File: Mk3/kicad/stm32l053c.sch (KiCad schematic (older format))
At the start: 24 parts, among them J1 CONN_01X02, P1 SWD, U1 AP2112, U2 STM32L053C8_LQFP48, U3 ADS1015, U4 EDGE_SMA, U5 RFM92/95

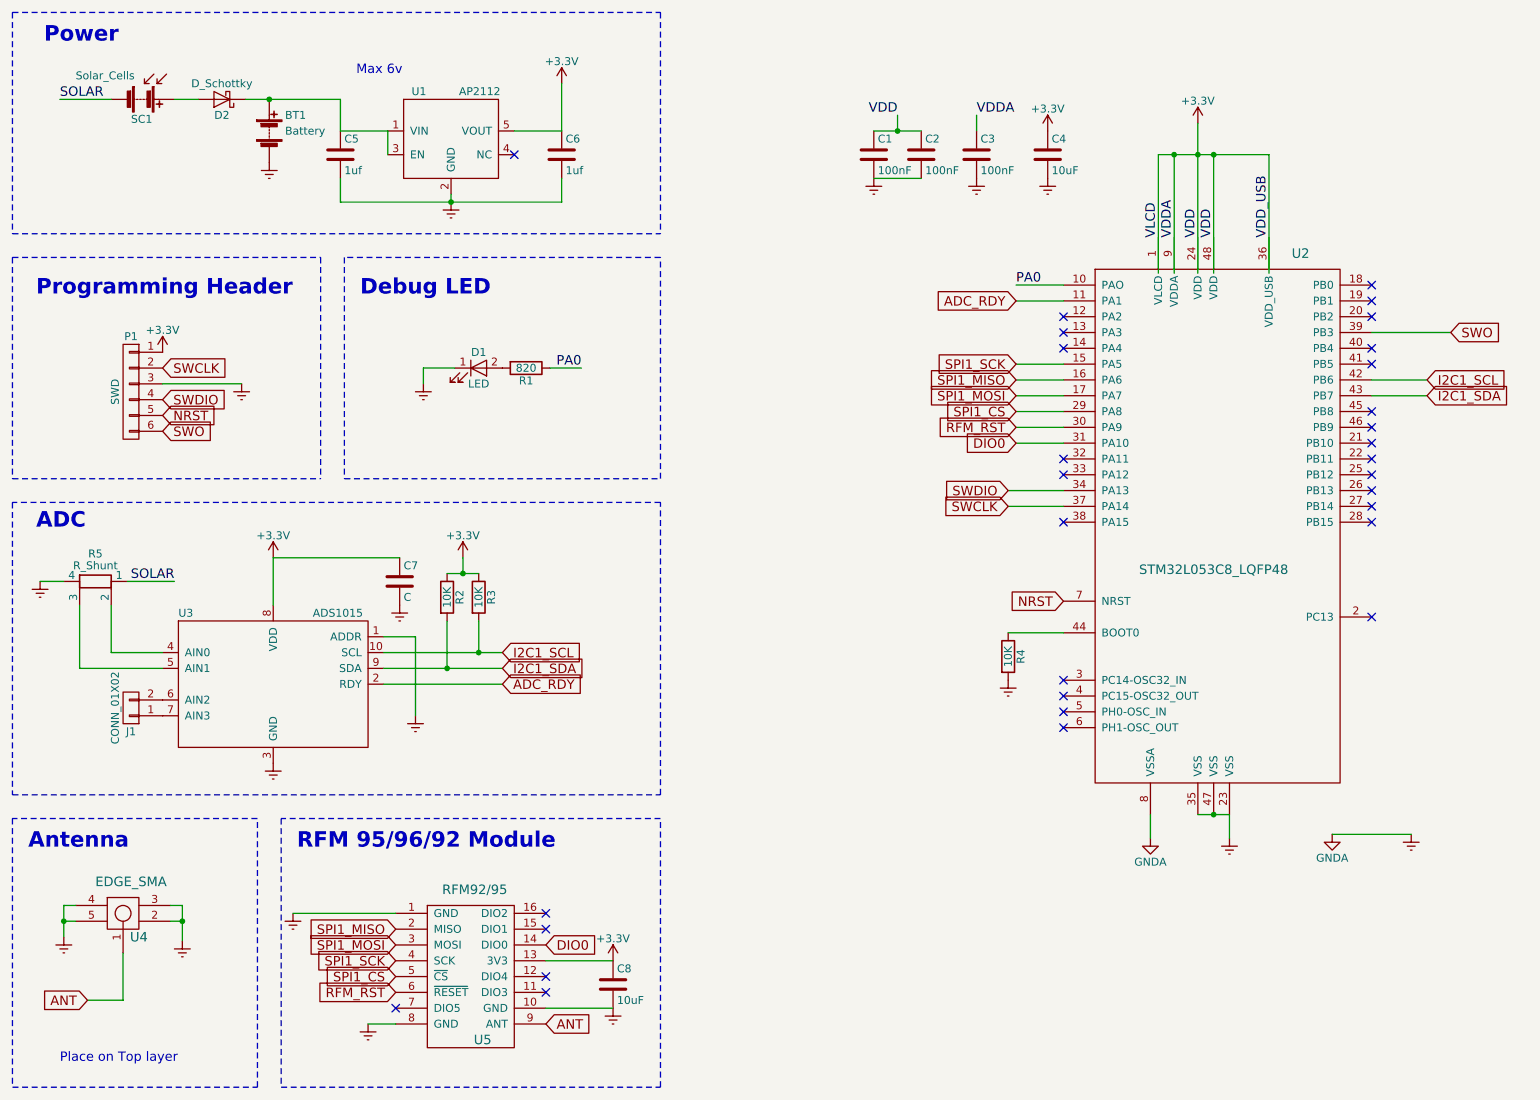
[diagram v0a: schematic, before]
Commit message: Solar power
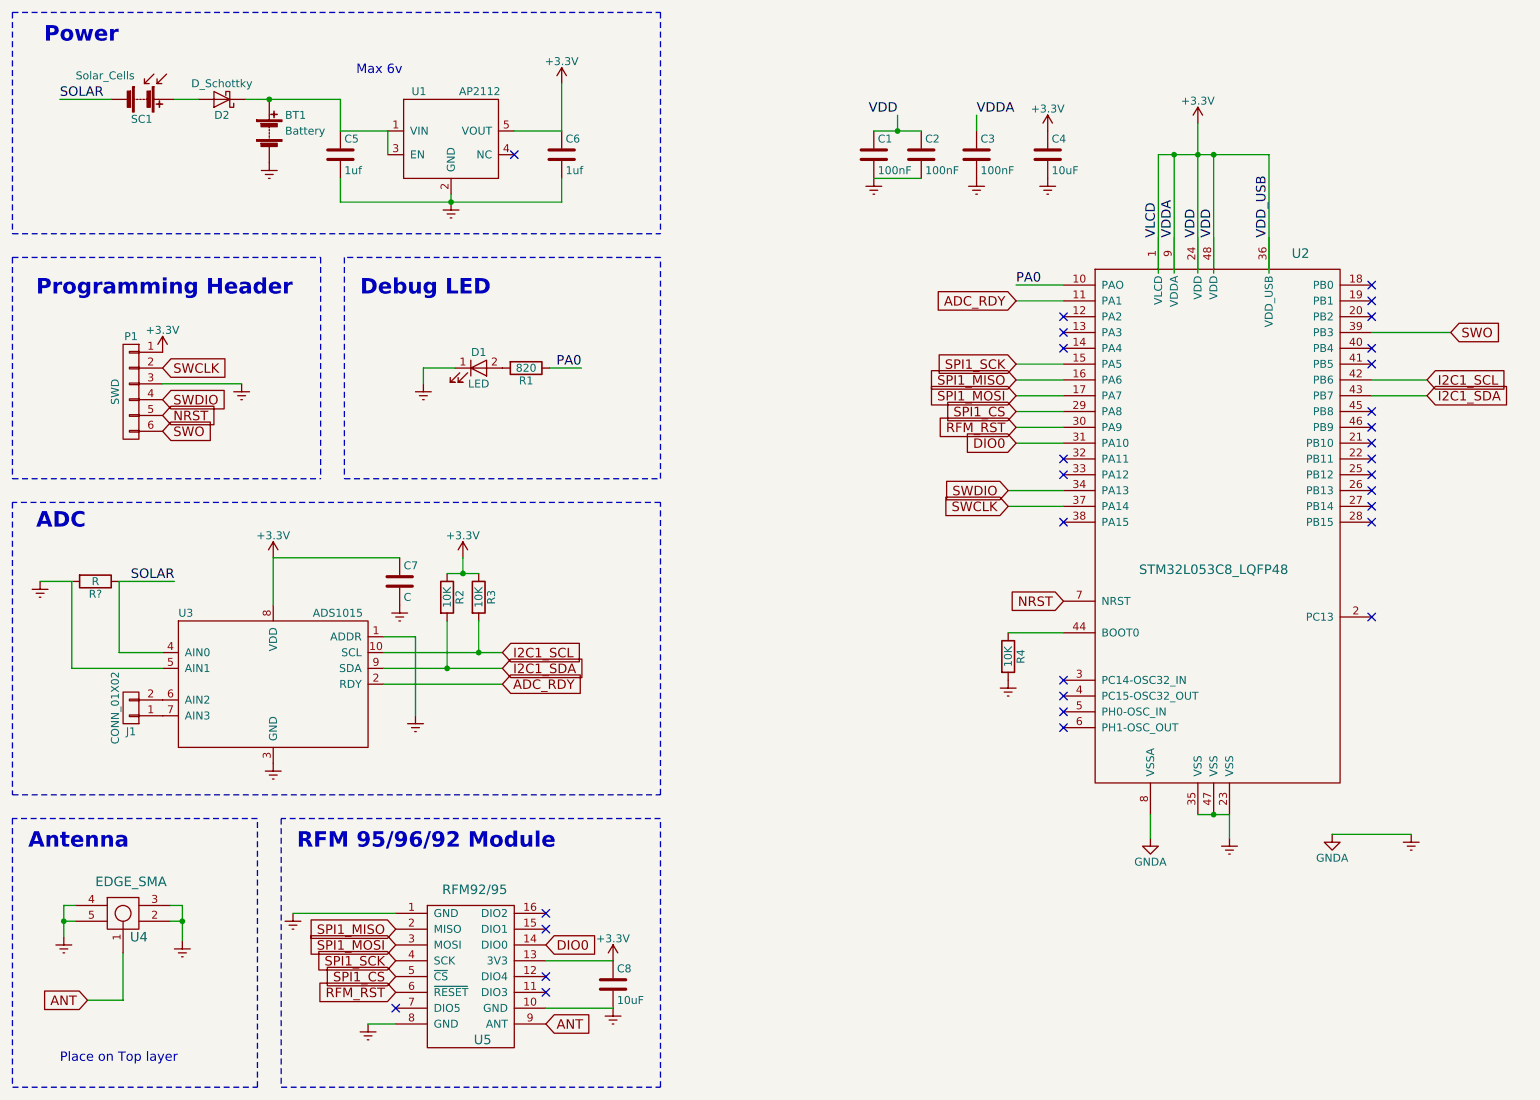
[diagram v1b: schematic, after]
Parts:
- removed R5: R_Shunt, symbol R_Shunt
- added R?: R, symbol R
- D2: footprint (none) -> Diodes_SMD:D_0805
- J1, SC1: footprint (none) -> Pin_Headers:Pin_Header_Straight_1x02_Pitch2.54mm
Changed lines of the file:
@@
 $EndDescr
 $Comp
-L Earth #PWR5
+L Earth #PWR01
 U 1 1 58021BE1
 P 6425 1775
-F 0 "#PWR5" H 6425 1525 50  0001 C CNN
+F 0 "#PWR01" H 6425 1525 50  0001 C CNN
 F 1 "Earth" H 6425 1625 50  0001 C CNN
 F 2 "" H 6425 1775 50  0000 C CNN
@@
 $EndComp
 $Comp
-L GNDA #PWR19
+L GNDA #PWR02
 U 1 1 58021F75
 P 9325 5925
-F 0 "#PWR19" H 9325 5675 50  0001 C CNN
+F 0 "#PWR02" H 9325 5675 50  0001 C CNN
 F 1 "GNDA" H 9325 5775 50  0000 C CNN
 F 2 "" H 9325 5925 50  0000 C CNN
@@
 $EndComp
 $Comp
-L Earth #PWR20
+L Earth #PWR03
 U 1 1 58021F89
 P 9825 5925
-F 0 "#PWR20" H 9825 5675 50  0001 C CNN
+F 0 "#PWR03" H 9825 5675 50  0001 C CNN
 F 1 "Earth" H 9825 5775 50  0001 C CNN
 F 2 "" H 9825 5925 50  0000 C CNN
@@
 $EndComp
 $Comp
-L GNDA #PWR21
+L GNDA #PWR04
 U 1 1 58022154
 P 8175 5950
-F 0 "#PWR21" H 8175 5700 50  0001 C CNN
+F 0 "#PWR04" H 8175 5700 50  0001 C CNN
 F 1 "GNDA" H 8175 5800 50  0000 C CNN
 F 2 "" H 8175 5950 50  0000 C CNN
@@
 $EndComp
 $Comp
-L Earth #PWR22
+L Earth #PWR05
 U 1 1 580221FA
 P 8675 5950
-F 0 "#PWR22" H 8675 5700 50  0001 C CNN
+F 0 "#PWR05" H 8675 5700 50  0001 C CNN
 F 1 "Earth" H 8675 5800 50  0001 C CNN
 F 2 "" H 8675 5950 50  0000 C CNN
@@
 $EndComp
 $Comp
-L Earth #PWR10
+L Earth #PWR06
 U 1 1 580369A9
 P 2425 3075
-F 0 "#PWR10" H 2425 2825 50  0001 C CNN
+F 0 "#PWR06" H 2425 2825 50  0001 C CNN
 F 1 "Earth" H 2425 2925 50  0001 C CNN
 F 2 "" H 2425 3075 50  0000 C CNN
@@
 PA0
 $Comp
-L Earth #PWR7
+L Earth #PWR07
 U 1 1 58039244
 P 7525 1775
-F 0 "#PWR7" H 7525 1525 50  0001 C CNN
+F 0 "#PWR07" H 7525 1525 50  0001 C CNN
 F 1 "Earth" H 7525 1625 50  0001 C CNN
 F 2 "" H 7525 1775 50  0000 C CNN
@@
 $EndComp
 $Comp
-L Earth #PWR6
+L Earth #PWR08
 U 1 1 5803BDC8
 P 7075 1775
-F 0 "#PWR6" H 7075 1525 50  0001 C CNN
+F 0 "#PWR08" H 7075 1525 50  0001 C CNN
 F 1 "Earth" H 7075 1625 50  0001 C CNN
 F 2 "" H 7075 1775 50  0000 C CNN
@@
 $EndComp
 $Comp
-L Earth #PWR16
+L Earth #PWR09
 U 1 1 58065816
 P 7275 4950
-F 0 "#PWR16" H 7275 4700 50  0001 C CNN
+F 0 "#PWR09" H 7275 4700 50  0001 C CNN
 F 1 "Earth" H 7275 4800 50  0001 C CNN
 F 2 "" H 7275 4950 50  0000 C CNN
@@
 $EndComp
 $Comp
-L Earth #PWR11
+L Earth #PWR010
 U 1 1 58077163
 P 3575 3075
-F 0 "#PWR11" H 3575 2825 50  0001 C CNN
+F 0 "#PWR010" H 3575 2825 50  0001 C CNN
 F 1 "Earth" H 3575 2925 50  0001 C CNN
 F 2 "" H 3575 3075 50  0000 C CNN
@@
 $EndComp
 $Comp
-L Earth #PWR18
+L Earth #PWR011
 U 1 1 592DF55A
 P 2625 5475
-F 0 "#PWR18" H 2625 5225 50  0001 C CNN
+F 0 "#PWR011" H 2625 5225 50  0001 C CNN
 F 1 "Earth" H 2625 5325 50  0001 C CNN
 F 2 "" H 2625 5475 50  0000 C CNN
@@
 NoConn ~ 4150 1625
 $Comp
-L Earth #PWR8
+L Earth #PWR012
 U 1 1 592F1C89
 P 3750 1925
-F 0 "#PWR8" H 3750 1675 50  0001 C CNN
+F 0 "#PWR012" H 3750 1675 50  0001 C CNN
 F 1 "Earth" H 3750 1775 50  0001 C CNN
 F 2 "" H 3750 1925 50  0000 C CNN
@@
 RFM_RST
 $Comp
-L +3.3V #PWR1
+L +3.3V #PWR013
 U 1 1 592F43A5
 P 4450 1175
-F 0 "#PWR1" H 4450 1025 50  0001 C CNN
+F 0 "#PWR013" H 4450 1025 50  0001 C CNN
 F 1 "+3.3V" H 4450 1315 50  0000 C CNN
 F 2 "" H 4450 1175 50  0001 C CNN
@@
 $EndComp
 $Comp
-L +3.3V #PWR9
+L +3.3V #PWR014
 U 1 1 592F4BC3
 P 1925 2875
-F 0 "#PWR9" H 1925 2725 50  0001 C CNN
+F 0 "#PWR014" H 1925 2725 50  0001 C CNN
 F 1 "+3.3V" H 1925 3015 50  0000 C CNN
 F 2 "" H 1925 2875 50  0001 C CNN
@@
 $EndComp
 $Comp
-L +3.3V #PWR2
+L +3.3V #PWR015
 U 1 1 592F4E66
 P 8475 1425
-F 0 "#PWR2" H 8475 1275 50  0001 C CNN
+F 0 "#PWR015" H 8475 1275 50  0001 C CNN
 F 1 "+3.3V" H 8475 1565 50  0000 C CNN
 F 2 "" H 8475 1425 50  0001 C CNN
@@
 $EndComp
 $Comp
-L +3.3V #PWR26
+L +3.3V #PWR016
 U 1 1 592F53D7
 P 4775 6725
-F 0 "#PWR26" H 4775 6575 50  0001 C CNN
+F 0 "#PWR016" H 4775 6575 50  0001 C CNN
 F 1 "+3.3V" H 4775 6865 50  0000 C CNN
 F 2 "" H 4775 6725 50  0001 C CNN
@@
 $EndComp
 $Comp
-L +3.3V #PWR3
+L +3.3V #PWR017
 U 1 1 592F54CD
 P 7525 1475
-F 0 "#PWR3" H 7525 1325 50  0001 C CNN
+F 0 "#PWR017" H 7525 1325 50  0001 C CNN
 F 1 "+3.3V" H 7525 1615 50  0000 C CNN
 F 2 "" H 7525 1475 50  0001 C CNN
@@
 NoConn ~ 3400 7025
 $Comp
-L Earth #PWR27
+L Earth #PWR018
 U 1 1 592F7C8A
 P 4775 7025
-F 0 "#PWR27" H 4775 6775 50  0001 C CNN
+F 0 "#PWR018" H 4775 6775 50  0001 C CNN
 F 1 "Earth" H 4775 6875 50  0001 C CNN
 F 2 "" H 4775 7025 50  0000 C CNN
@@
 $EndComp
 $Comp
-L Earth #PWR23
+L Earth #PWR019
 U 1 1 592F7CF0
 P 2750 6425
-F 0 "#PWR23" H 2750 6175 50  0001 C CNN
+F 0 "#PWR019" H 2750 6175 50  0001 C CNN
 F 1 "Earth" H 2750 6275 50  0001 C CNN
 F 2 "" H 2750 6425 50  0000 C CNN
@@
 $EndComp
 $Comp
-L Earth #PWR28
+L Earth #PWR020
 U 1 1 592F7EE4
 P 3225 7125
-F 0 "#PWR28" H 3225 6875 50  0001 C CNN
+F 0 "#PWR020" H 3225 6875 50  0001 C CNN
 F 1 "Earth" H 3225 6975 50  0001 C CNN
 F 2 "" H 3225 7125 50  0000 C CNN
@@
 $EndComp
 $Comp
-L Earth #PWR24
+L Earth #PWR021
 U 1 1 592F80DC
 P 1300 6575
-F 0 "#PWR24" H 1300 6325 50  0001 C CNN
+F 0 "#PWR021" H 1300 6325 50  0001 C CNN
 F 1 "Earth" H 1300 6425 50  0001 C CNN
 F 2 "" H 1300 6575 50  0000 C CNN
@@
 $EndComp
 $Comp
-L Earth #PWR25
+L Earth #PWR022
 U 1 1 592F814F
 P 2050 6600
-F 0 "#PWR25" H 2050 6350 50  0001 C CNN
+F 0 "#PWR022" H 2050 6350 50  0001 C CNN
 F 1 "Earth" H 2050 6450 50  0001 C CNN
 F 2 "" H 2050 6600 50  0000 C CNN
@@
 $EndComp
 $Comp
-L Earth #PWR17
+L Earth #PWR023
 U 1 1 59301904
 P 3525 5175
-F 0 "#PWR17" H 3525 4925 50  0001 C CNN
+F 0 "#PWR023" H 3525 4925 50  0001 C CNN
 F 1 "Earth" H 3525 5025 50  0001 C CNN
 F 2 "" H 3525 5175 50  0000 C CNN
@@
 $EndComp
 $Comp
-L Earth #PWR15
+L Earth #PWR024
 U 1 1 593024E3
 P 3425 4475
-F 0 "#PWR15" H 3425 4225 50  0001 C CNN
+F 0 "#PWR024" H 3425 4225 50  0001 C CNN
 F 1 "Earth" H 3425 4325 50  0001 C CNN
 F 2 "" H 3425 4475 50  0000 C CNN
@@
 $EndComp
 $Comp
-L +3.3V #PWR12
+L +3.3V #PWR025
 U 1 1 59303669
 P 2625 4175
-F 0 "#PWR12" H 2625 4025 50  0001 C CNN
+F 0 "#PWR025" H 2625 4025 50  0001 C CNN
 F 1 "+3.3V" H 2625 4315 50  0000 C CNN
 F 2 "" H 2625 4175 50  0001 C CNN
@@
 $EndComp
 $Comp
-L +3.3V #PWR13
+L +3.3V #PWR026
 U 1 1 59303771
 P 3825 4175
-F 0 "#PWR13" H 3825 4025 50  0001 C CNN
+F 0 "#PWR026" H 3825 4025 50  0001 C CNN
 F 1 "+3.3V" H 3825 4315 50  0000 C CNN
 F 2 "" H 3825 4175 50  0001 C CNN
@@
 $EndComp
 $Comp
-L Earth #PWR4
+L Earth #PWR027
 U 1 1 59316863
 P 2600 1675
-F 0 "#PWR4" H 2600 1425 50  0001 C CNN
+F 0 "#PWR027" H 2600 1425 50  0001 C CNN
 F 1 "Earth" H 2600 1525 50  0001 C CNN
 F 2 "" H 2600 1675 50  0000 C CNN
@@
 F 0 "SC1" V 1925 1200 50  0000 L CNN
 F 1 "Solar_Cells" V 1650 850 50  0000 L CNN
-F 2 "" V 1800 1335 50  0001 C CNN
+F 2 "Pin_Headers:Pin_Header_Straight_1x02_Pitch2.54mm" V 1800 1335 50  0001 C CNN
 F 3 "" V 1800 1335 50  0001 C CNN
 	1    1800 1275
@@
 F 0 "D2" H 2300 1375 50  0000 C CNN
 F 1 "D_Schottky" H 2300 1175 50  0000 C CNN
-F 2 "" H 2300 1275 50  0001 C CNN
+F 2 "Diodes_SMD:D_0805" H 2300 1275 50  0001 C CNN
 F 3 "" H 2300 1275 50  0001 C CNN
 	1    2300 1275
@@
 $EndComp
 $Comp
-L R_Shunt R5
-U 1 1 59328FA3
-P 1500 4325
-F 0 "R5" V 1325 4325 50  0000 C CNN
-F 1 "R_Shunt" V 1400 4325 50  0000 C CNN
-F 2 "" V 1430 4325 50  0001 C CNN
-F 3 "" H 1500 4325 50  0001 C CNN
-	1    1500 4325
-	0    1    1    0
-$EndComp
-$Comp
-L Earth #PWR14
+L Earth #PWR028
 U 1 1 593290F6
 P 1150 4325
-F 0 "#PWR14" H 1150 4075 50  0001 C CNN
+F 0 "#PWR028" H 1150 4075 50  0001 C CNN
 F 1 "Earth" H 1150 4175 50  0001 C CNN
 F 2 "" H 1150 4325 50  0000 C CNN
@@
 Connection ~ 8575 1625
 Wire Wire Line
-	6725 1475 6425 1475
+	6425 1475 6725 1475
 Wire Wire Line
 	6725 1775 6425 1775
@@
 F 0 "J1" H 1725 5275 50  0000 C CNN
 F 1 "CONN_01X02" V 1825 5125 50  0000 C CNN
-F 2 "" H 1725 5125 50  0001 C CNN
+F 2 "Pin_Headers:Pin_Header_Straight_1x02_Pitch2.54mm" H 1725 5125 50  0001 C CNN
 F 3 "" H 1725 5125 50  0001 C CNN
 	1    1725 5125
@@
 SOLAR
 Wire Wire Line
-	1700 4325 2000 4325
-Wire Wire Line
-	1300 4325 1150 4325
-Wire Wire Line
-	1600 4475 1600 4775
-Wire Wire Line
-	1600 4775 1925 4775
-Wire Wire Line
-	1925 4875 1400 4875
-Wire Wire Line
-	1400 4875 1400 4475
+	1650 4325 2000 4325
+Wire Wire Line
+	1350 4325 1150 4325
+Wire Wire Line
+	1650 4325 1650 4775
+Wire Wire Line
+	1650 4775 1925 4775
+Wire Wire Line
+	1350 4875 1925 4875
+Wire Wire Line
+	1350 4325 1350 4875
 Text Label 1275 1275 0    60   ~ 0
 SOLAR
@@
 	1    0    0    -1
 $EndComp
+$Comp
+L R R?
+U 1 1 59340973
+P 1500 4325
+F 0 "R?" V 1580 4325 50  0000 C CNN
+F 1 "R" V 1500 4325 50  0000 C CNN
+F 2 "" V 1430 4325 50  0001 C CNN
+F 3 "" H 1500 4325 50  0001 C CNN
+	1    1500 4325
+	0    1    1    0
+$EndComp
 $EndSCHEMATC
